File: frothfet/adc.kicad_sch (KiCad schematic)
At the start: 16 parts, among them U25 MCP3564R

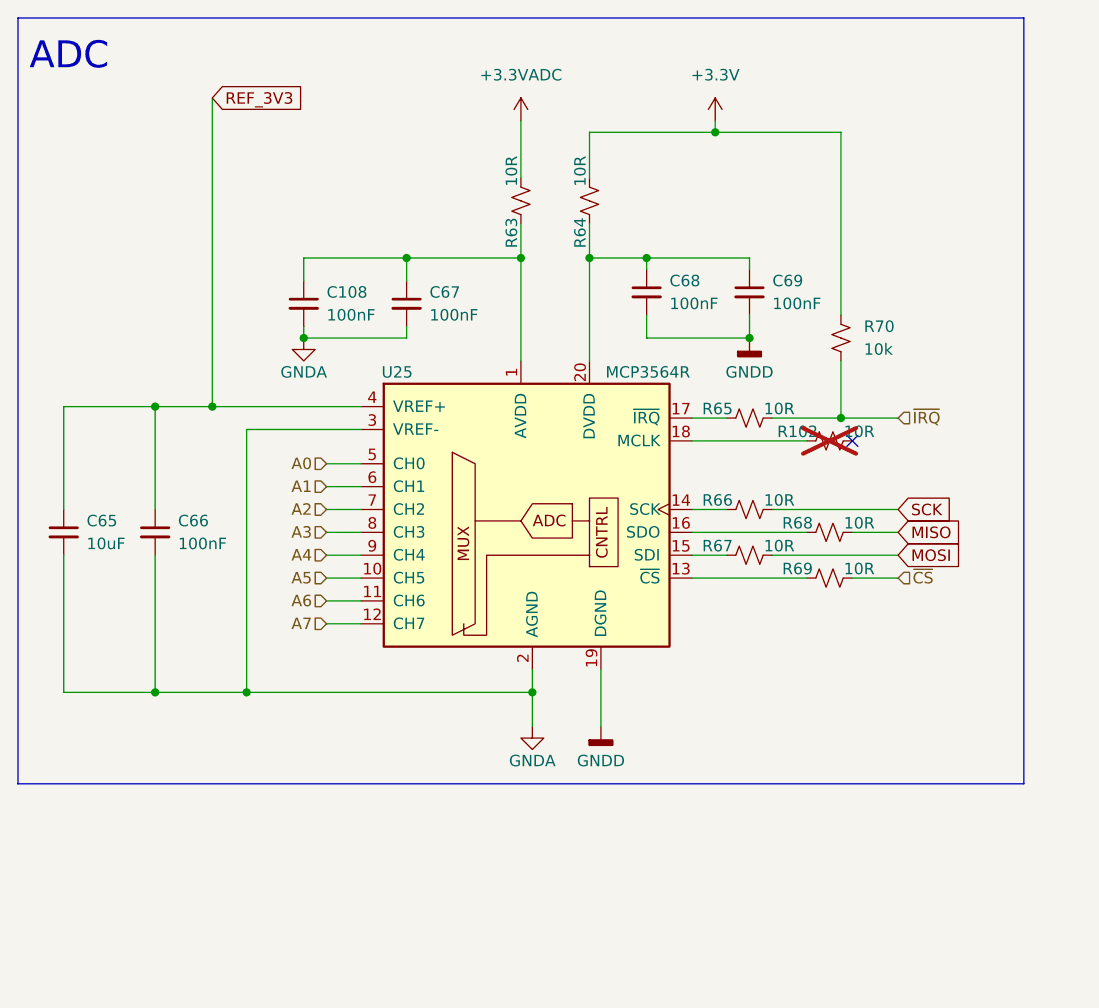
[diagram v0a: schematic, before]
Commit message: lots of work on the analog system
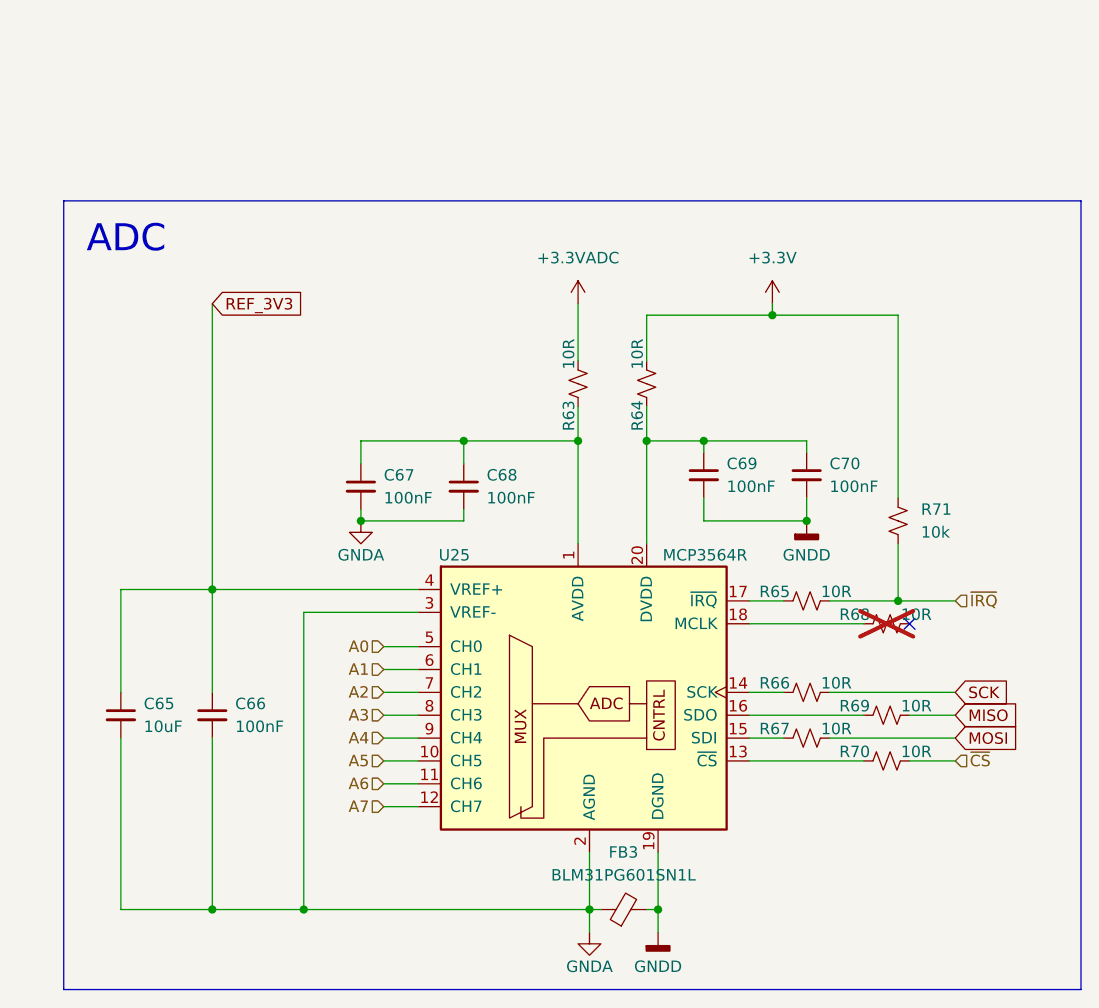
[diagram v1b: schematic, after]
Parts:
- added FB3: BLM31PG601SN1L, Inductor_SMD:L_1206_3216Metric, symbol Device:FerriteBead_Small
- renumbered C108 to C67, C67 to C68, C68 to C69, C69 to C70, R102 to R68, R68 to R69, R69 to R70, R70 to R71
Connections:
- net GNDA: now also FB3.1
- net GNDD: now also FB3.2
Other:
- moved on the sheet: C65, C66, C67, C68, C69, C70, R63, R64, R65, R66, R67, R68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
